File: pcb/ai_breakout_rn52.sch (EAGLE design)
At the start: 8 parts, among them J1 1X20, J2 1X20

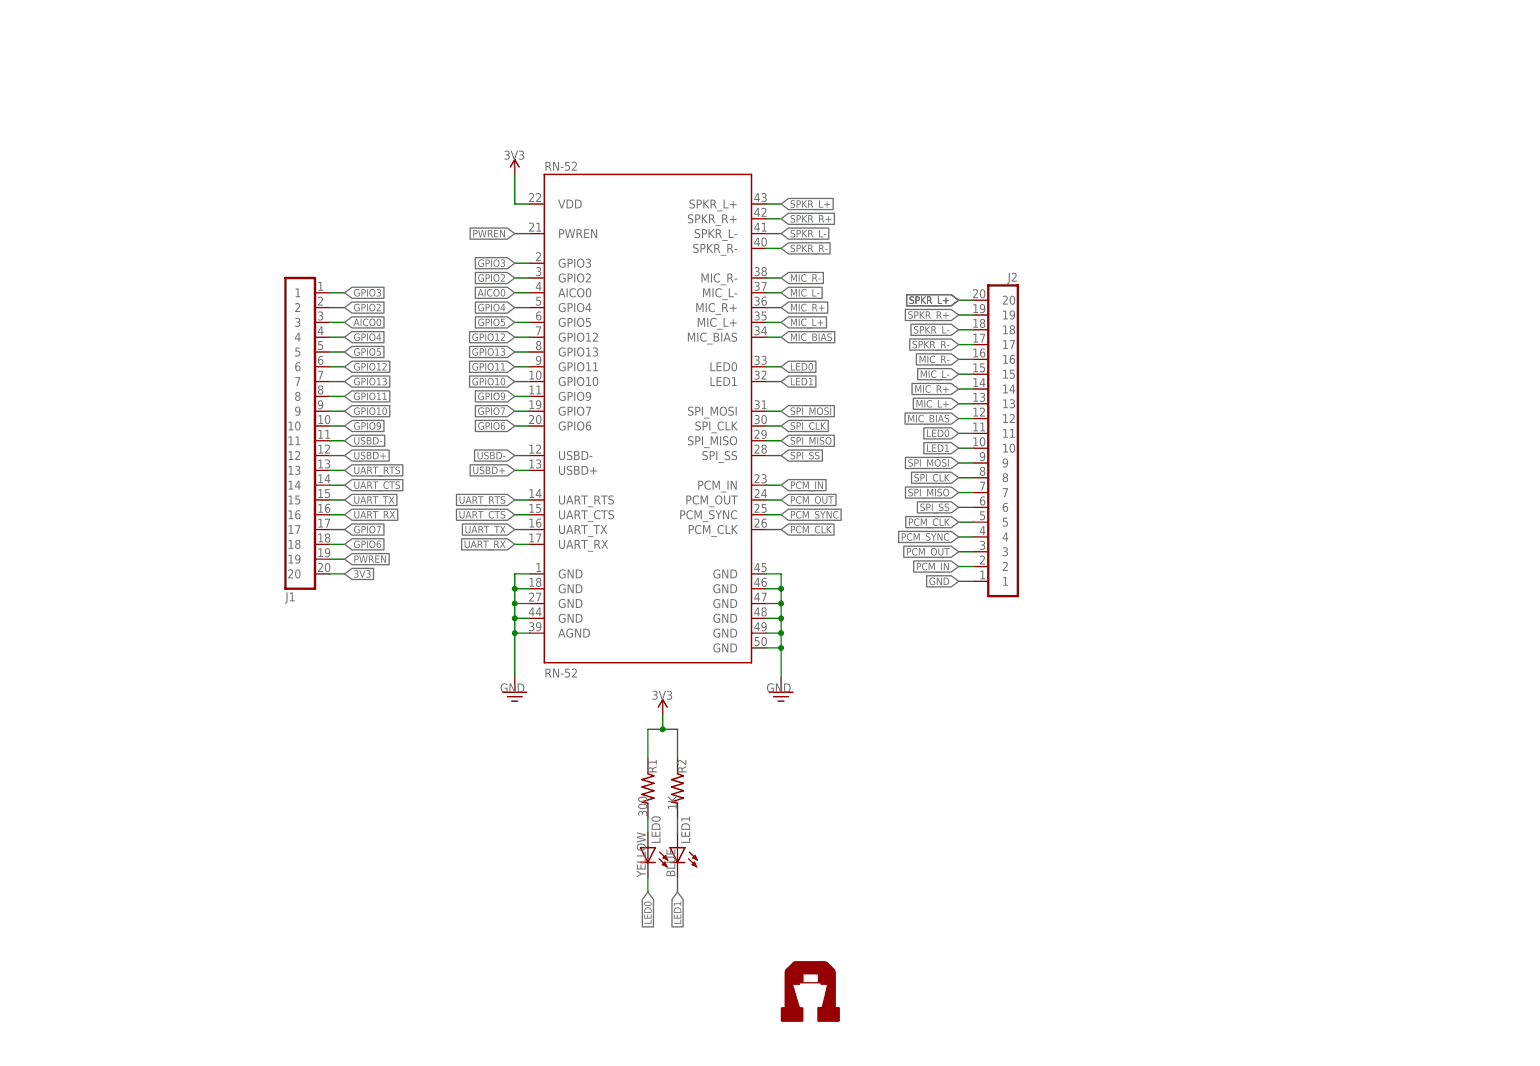
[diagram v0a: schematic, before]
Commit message: updating
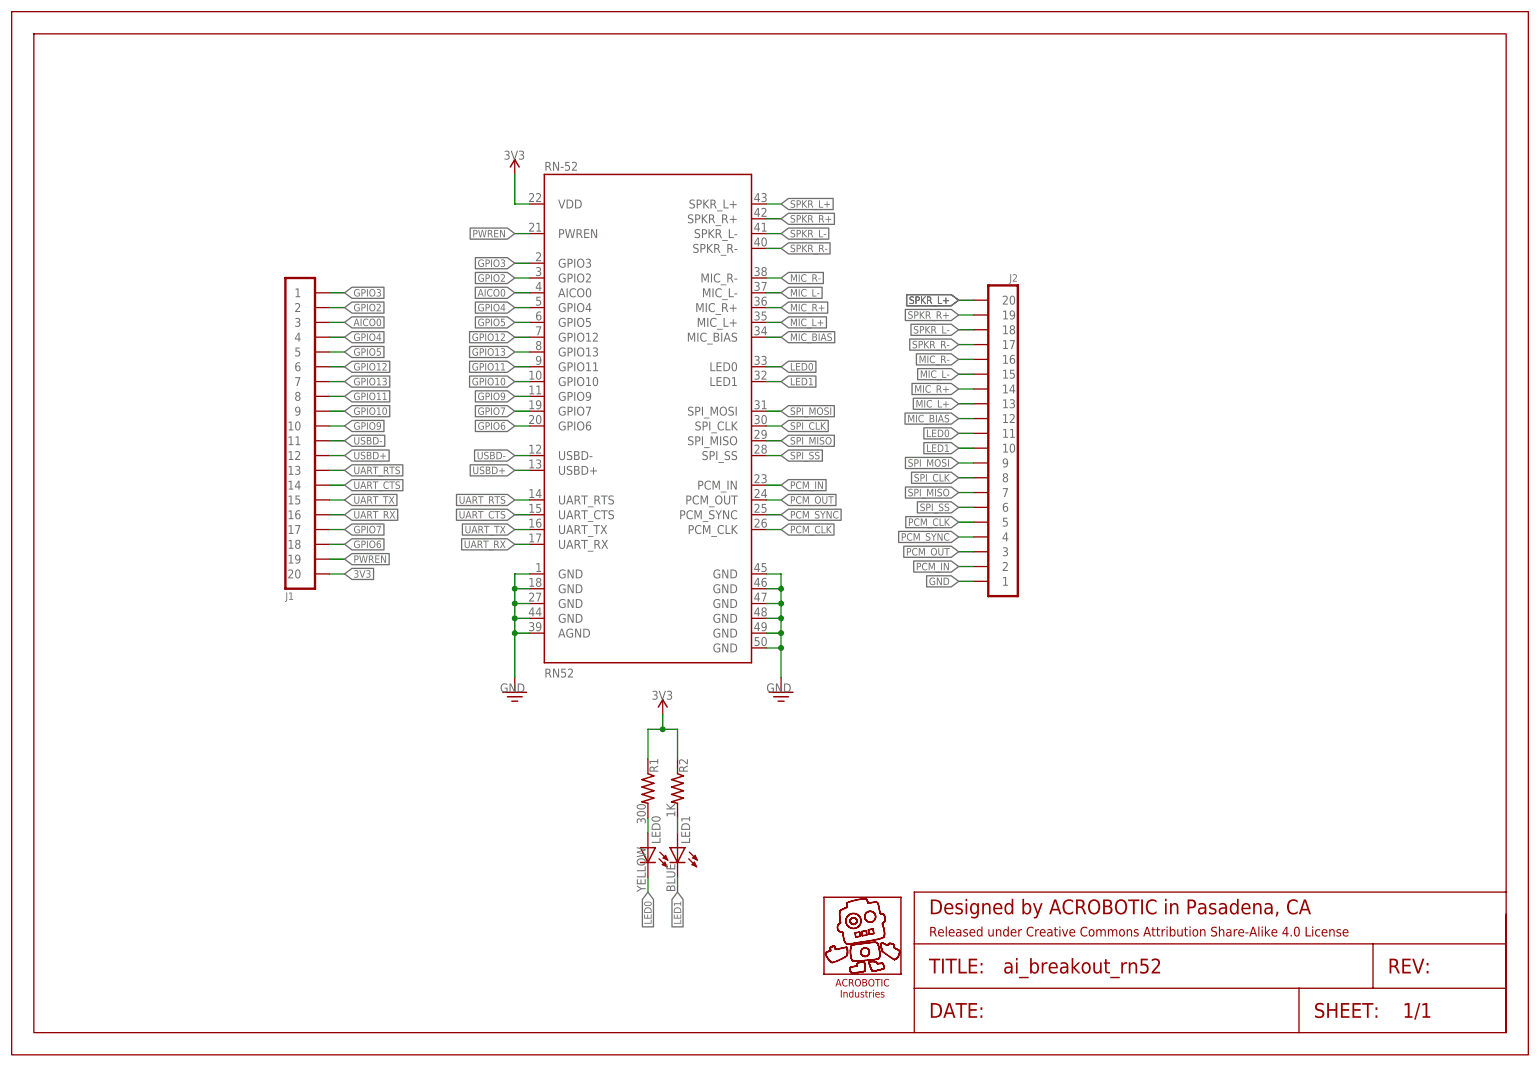
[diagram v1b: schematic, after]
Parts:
- added FRAME1: FRAME-LETTER, Ai_Miscellany:FRAME-LETTER
- RN-52: value RN-52 -> RN52; device Ai_IC:RN-52 -> Ai_RF:RN52
- U$3: value AI-LOGOL -> AI-LOGOXS; device Ai_Miscellany:AI-LOGOL -> Ai_Miscellany:AI-LOGOXS
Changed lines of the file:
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@@
 <?xml version="1.0" encoding="utf-8"?>
 <!DOCTYPE eagle SYSTEM "eagle.dtd">
-<eagle version="6.5.0">
+<eagle version="7.1.0">
 <drawing>
 <settings>
@@
 <setting verticaltext="up"/>
 </settings>
-<grid distance="0.1" unitdist="inch" unit="inch" style="lines" multiple="1" display="no" altdistance="0.01" altunitdist="inch" altunit="inch"/>
+<grid distance="50" unitdist="mil" unit="mil" style="lines" multiple="1" display="yes" altdistance="0.01" altunitdist="inch" altunit="inch"/>
 <layers>
 <layer number="1" name="Top" color="4" fill="1" visible="no" active="no"/>
@@
 <layer number="56" name="wert" color="7" fill="1" visible="no" active="no"/>
 <layer number="57" name="tCAD" color="7" fill="1" visible="no" active="no"/>
+<layer number="59" name="tCarbon" color="7" fill="1" visible="no" active="no"/>
+<layer number="60" name="bCarbon" color="7" fill="1" visible="no" active="no"/>
+<layer number="90" name="Modules" color="5" fill="1" visible="yes" active="yes"/>
 <layer number="91" name="Nets" color="2" fill="1" visible="yes" active="yes"/>
 <layer number="92" name="Busses" color="1" fill="1" visible="yes" active="yes"/>
@@
 <layer number="97" name="Info" color="7" fill="1" visible="yes" active="yes"/>
 <layer number="98" name="Guide" color="6" fill="1" visible="yes" active="yes"/>
+<layer number="99" name="SpiceOrder" color="7" fill="1" visible="no" active="no"/>
 <layer number="100" name="Muster" color="7" fill="1" visible="no" active="no"/>
 <layer number="101" name="Patch_Top" color="12" fill="4" visible="yes" active="yes"/>
@@
 <layer number="112" name="tSilk" color="7" fill="1" visible="yes" active="yes"/>
 <layer number="113" name="Route13" color="7" fill="1" visible="no" active="no"/>
+<layer number="114" name="Badge_Outline" color="7" fill="1" visible="yes" active="yes"/>
+<layer number="115" name="ReferenceISLANDS" color="7" fill="1" visible="yes" active="yes"/>
 <layer number="116" name="Patch_BOT" color="9" fill="4" visible="yes" active="yes"/>
 <layer number="117" name="mPads" color="7" fill="1" visible="no" active="no"/>
@@
 <layer number="223" name="223bmp" color="24" fill="1" visible="no" active="no"/>
 <layer number="224" name="224bmp" color="25" fill="1" visible="no" active="no"/>
+<layer number="225" name="225bmp" color="7" fill="1" visible="yes" active="yes"/>
+<layer number="226" name="226bmp" color="7" fill="1" visible="yes" active="yes"/>
+<layer number="227" name="227bmp" color="7" fill="1" visible="yes" active="yes"/>
+<layer number="228" name="228bmp" color="7" fill="1" visible="yes" active="yes"/>
+<layer number="229" name="229bmp" color="7" fill="1" visible="yes" active="yes"/>
+<layer number="230" name="230bmp" color="7" fill="1" visible="yes" active="yes"/>
+<layer number="231" name="231bmp" color="7" fill="1" visible="yes" active="yes"/>
 <layer number="248" name="Housing" color="7" fill="1" visible="yes" active="yes"/>
 <layer number="249" name="Edge" color="7" fill="1" visible="yes" active="yes"/>
@@
 <layer number="251" name="SMDround" color="7" fill="1" visible="no" active="no"/>
 <layer number="254" name="cooling" color="7" fill="1" visible="yes" active="yes"/>
+<layer number="255" name="routoute" color="7" fill="1" visible="yes" active="yes"/>
 </layers>
 <schematic xreflabel="%F%N/%S.%C%R" xrefpart="/%S.%C%R">
@@
 <parts>
 <part name="FRAME1" library="Ai_Miscellany" deviceset="FRAME-LETTER" device="">
-<attribute name="AUTHOR" value="A.I. HARDWARE SITH LORDS"/>
-<attribute name="REV" value="1.0"/>
+<attribute name="REV" value="1.1"/>
 </part>
 <part name="LED0" library="Ai_LED" deviceset="LED" device="0603" value="YELLOW"/>
@@
 <part name="J2" library="Ai_Connectors" deviceset="1X20" device=""/>
 <part name="J1" library="Ai_Connectors" deviceset="1X20" device=""/>
-<part name="RN-52" library="Ai_IC" deviceset="RN-52" device=""/>
+<part name="RN-52" library="Ai_RF" deviceset="RN52" device=""/>
 <part name="GND1" library="Ai_Power" deviceset="GND" device=""/>
 <part name="GND2" library="Ai_Power" deviceset="GND" device=""/>
-<part name="U$3" library="Ai_Miscellany" deviceset="AI-LOGO" device="L"/>
+<part name="U$3" library="Ai_Miscellany" deviceset="AI-LOGO" device="XS" value="AI-LOGOXS"/>
 </parts>
 <sheets>
@@
 <instances>
 <instance part="FRAME1" gate="G$1" x="0" y="0"/>
-<instance part="FRAME1" gate="G$2" x="147.32" y="0">
-<attribute name="AUTHOR" x="147.32" y="0" size="1.778" layer="96" display="off"/>
-<attribute name="REV" x="147.32" y="0" size="1.778" layer="96" display="off"/>
+<instance part="FRAME1" gate="G$2" x="154.94" y="3.81">
+<attribute name="REV" x="154.94" y="3.81" size="1.778" layer="96" display="off"/>
 </instance>
 <instance part="LED0" gate="G$1" x="109.22" y="35.56" rot="MR0"/>
@@
 <instance part="GND1" gate="GND" x="132.08" y="62.23"/>
 <instance part="GND2" gate="GND" x="86.36" y="62.23"/>
-<instance part="U$3" gate="G$1" x="137.16" y="10.16"/>
+<instance part="U$3" gate="G$1" x="146.05" y="19.05"/>
 </instances>
 <busses>
@@
 </schematic>
 </drawing>
+<compatibility>
+<note version="6.3" minversion="6.2.2" severity="warning">
+Since Version 6.2.2 text objects can contain more than one line,
+which will not be processed correctly with this version.
+</note>
+</compatibility>
 </eagle>
